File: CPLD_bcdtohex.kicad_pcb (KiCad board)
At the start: 2 copper layers, 27 x 90.1 mm, 5 parts, among them IC1 ATF750C-10PU, J1 Conn_01x08_Pin

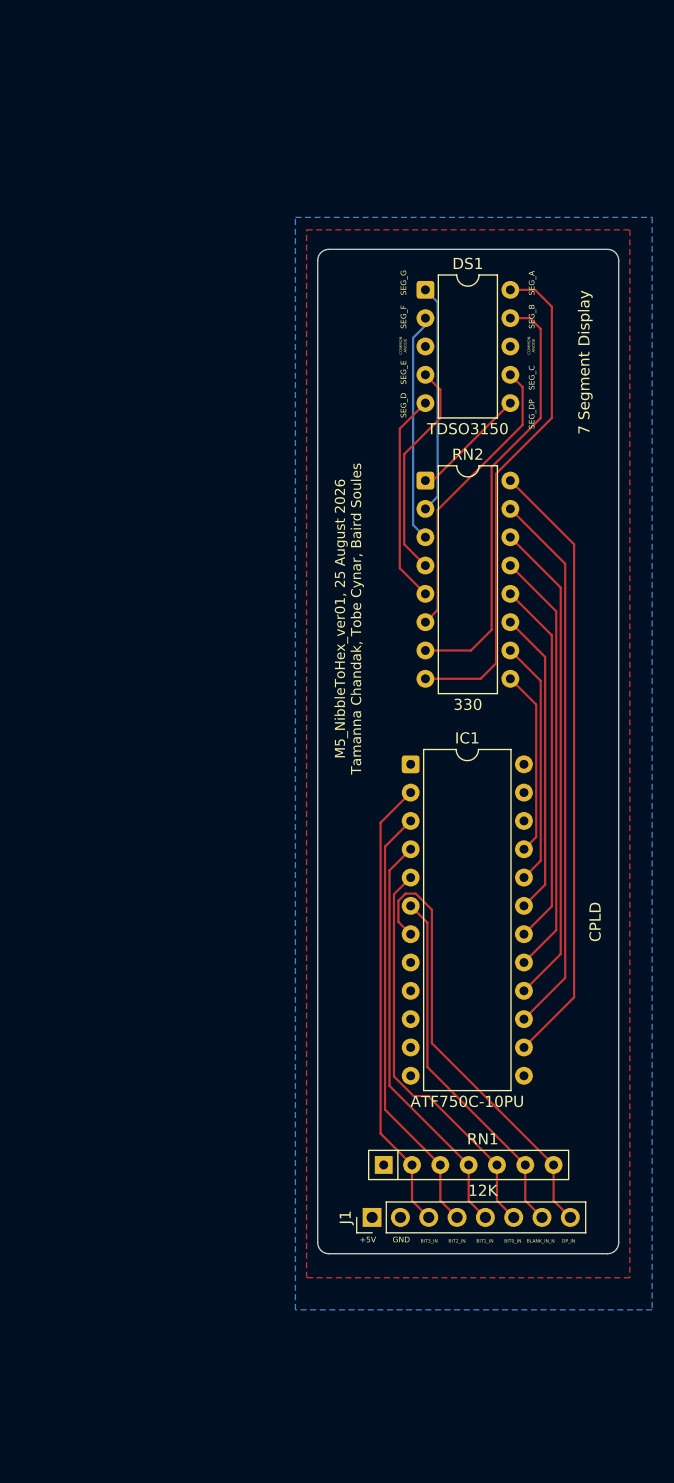
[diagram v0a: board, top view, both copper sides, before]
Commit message: PCB RevA
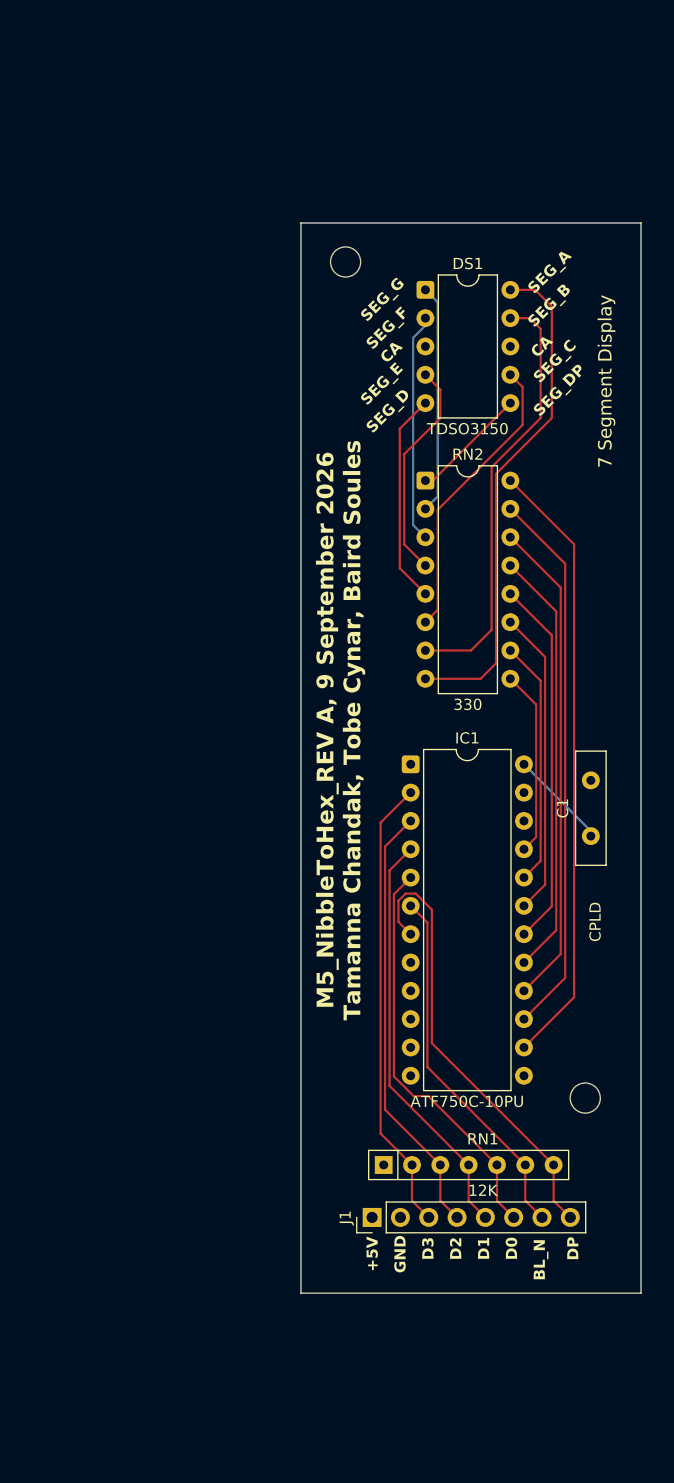
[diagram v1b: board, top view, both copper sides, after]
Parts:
- added C1: 0.1µF, Capacitor_THT:C_Disc_D10.0mm_W2.5mm_P5.00mm, F.Cu at (163.5, 114.5)
- added mh: MountingHole_2.7mm_M2.5, MountingHole:MountingHole_2.7mm_M2.5, F.Cu at (163.0, 138.0)
- added mh: MountingHole_2.7mm_M2.5, MountingHole:MountingHole_2.7mm_M2.5, F.Cu at (141.5, 63.0)
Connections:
- net /BIT1_IN renamed /D1
- net /BIT3_IN renamed /D3
- net /BLANK_IN_N renamed /BLANK
- net /DP_IN renamed /DP
- IC1 pad 24: +5V -> Net-(IC1-VCC)
- IC1 pad 3: /BIT2_IN -> /D2
- IC1 pad 5: /BIT2_IN -> /D0
- J1 pad 4: /BIT2_IN -> /D2
- J1 pad 6: /BIT2_IN -> /D0
- RN1 pad 3: /BIT2_IN -> /D2
- RN1 pad 5: /BIT2_IN -> /D0
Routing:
- net /BIT2_IN: track 75.6 -> 0.00 mm
- net /D2: track 0.00 -> 39.2 mm
- net /D0: track 0.00 -> 36.4 mm
- net Net-(IC1-VCC): track 0.00 -> 8.93 mm
- added copper zone on In1.Cu, net +5V
- added copper zone on In2.Cu, net GND
- removed copper zone on F.Cu, net +5V
- removed copper zone on B.Cu, net GND
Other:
- board size 27 x 90.1 mm -> 30.5 x 96 mm
- copper layers 2 -> 4
- board text added: "BL_N"
- board text added: "CA"
- board text added: "D0"
- board text added: "D1"
- board text added: "D2"
- board text added: "D3"
- board text added: "DP"
- board text added: "M5_NibbleToHex_REV A, 9 September 2026 Tamanna Chandak, Tobe Cynar, Baird Soules"
- board text added: "https://www.umassamherstm5.org/blog/m5hexdisplay"
- board text removed: "BIT0_IN"
- board text removed: "BIT1_IN"
- board text removed: "BIT2_IN"
- board text removed: "BIT3_IN"
- board text removed: "BLANK_IN_N"
- board text removed: "COMMON ANODE"
- board text removed: "DP_IN"
- board text removed: "M5_NibbleToHex_ver01, 25 August 2026 Tamanna Chandak, Tobe Cynar, Baird Soules"

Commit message: v0.5
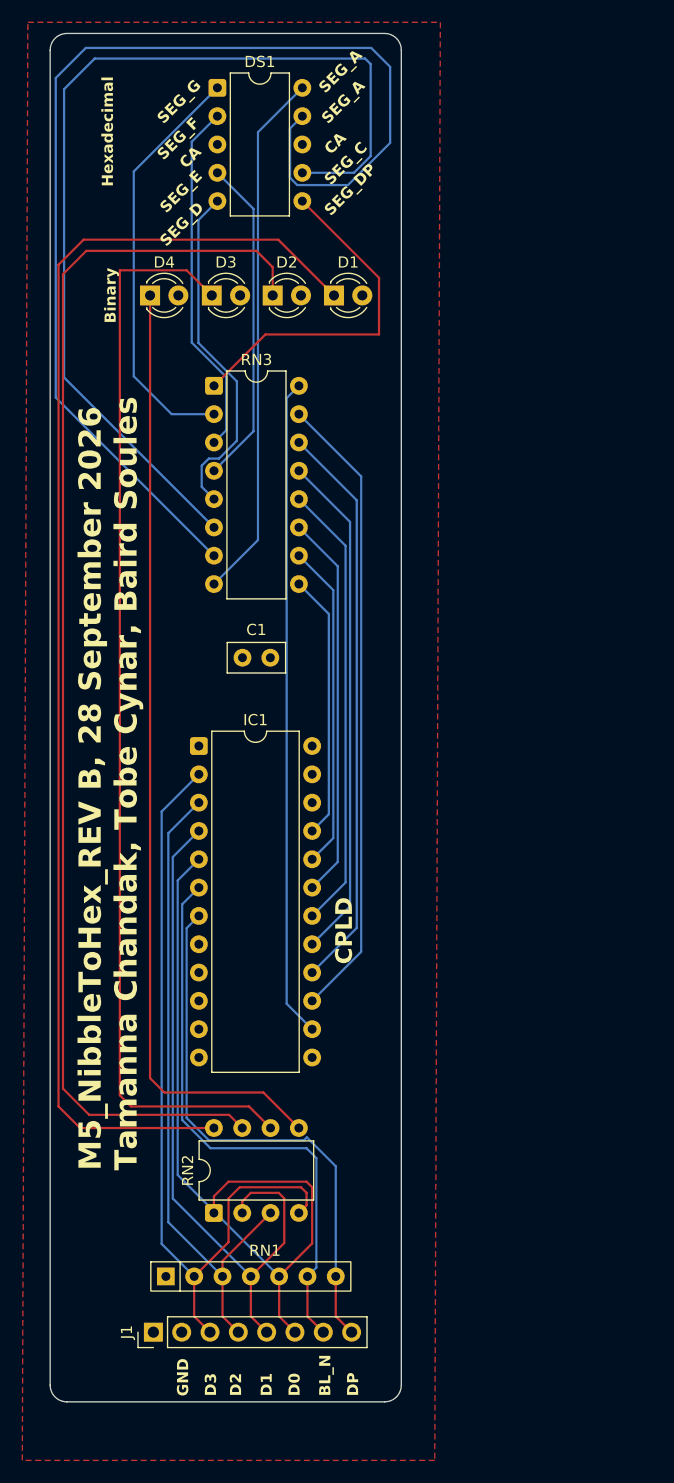
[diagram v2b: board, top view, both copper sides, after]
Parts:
- removed mh (x2): MountingHole_2.7mm_M2.5, MountingHole:MountingHole_2.7mm_M2.5
- added D1: LED, LED_THT:LED_D3.0mm, F.Cu at (140.5, 66.0)
- added D2: LED, LED_THT:LED_D3.0mm, F.Cu at (135.0, 66.0)
- added D3: LED, LED_THT:LED_D3.0mm, F.Cu at (129.5, 66.0)
- added D4: LED, LED_THT:LED_D3.0mm, F.Cu at (124.0, 66.0)
- added RN3: 330, Package_DIP:DIP-16_W7.62mm, F.Cu at (129.7, 74.1)
- C1: footprint Capacitor_THT:C_Disc_D10.0mm_W2.5mm_P5.00mm -> Capacitor_THT:C_Disc_D5.0mm_W2.5mm_P2.50mm
- RN1: value 12K -> 10K
- RN2: value 330 -> 220; footprint Package_DIP:DIP-16_W7.62mm -> Package_DIP:DIP-8_W7.62mm
- moved RN2 68.4 mm to (129.7, 148.3), turned to 90 degrees
- moved C1 35.1 mm to (132.2, 98.5), turned to 0 degrees
- moved DS1 26.0 mm to (130.0, 47.4)
- moved J1 22.2 mm to (124.3, 159.0)
- moved RN1 22.0 mm to (125.4, 154.0)
- moved IC1 19.1 mm to (128.3, 106.4)
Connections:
- net /BLANK renamed /BLANK_N
- C1 pad 1: Net-(IC1-VCC) -> +5V
- IC1 pad 24: Net-(IC1-VCC) -> +5V
- RN2 pad 1: Net-(DS1-DP) -> /D0
- RN2 pad 2: Net-(DS1-g) -> /D1
- RN2 pad 3: Net-(DS1-f) -> /D2
- RN2 pad 4: Net-(DS1-e) -> /D3
- RN2 pad 5: Net-(DS1-d) -> Net-(D4-K)
- RN2 pad 6: Net-(DS1-c) -> Net-(D3-K)
- RN2 pad 7: Net-(DS1-b) -> Net-(D2-K)
- RN2 pad 8: Net-(DS1-a) -> Net-(D1-K)
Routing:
- net Net-(D1-K): track 0.00 -> 118.0 mm
- net Net-(D2-K): track 0.00 -> 113.4 mm
- net Net-(D3-K): track 0.00 -> 97.9 mm
- net Net-(D4-K): track 0.00 -> 85.4 mm
- net Net-(DS1-b): track 38.6 -> 104.2 mm
- net Net-(DS1-c): track 26.3 -> 88.7 mm
- net /D0: track 36.4 -> 67.8 mm
- net /D3: track 41.0 -> 71.2 mm
- net /D1: track 37.4 -> 63.0 mm
- net Net-(DS1-DP): track 10.5 -> 31.5 mm
- net /D2: track 39.2 -> 58.7 mm
- net /BLANK_N: track 32.8 -> 51.5 mm
- net Net-(DS1-g): track 20.6 -> 37.6 mm
- net Net-(DS1-d): track 19.0 -> 31.2 mm
- net Net-(DS1-f): track 21.6 -> 32.0 mm
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- added copper zone on F.Cu, net +5V
- removed copper zone on In1.Cu, net +5V
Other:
- board size 30.5 x 96 mm -> 31.5 x 122.8 mm
- board text added: "Binary"
- board text added: "Hexadecimal"
- board text added: "M5_NibbleToHex_REV B, 28 September 2026 Tamanna Chandak, Tobe Cynar, Baird Soules"
- board text removed: "+5V"
- board text removed: "7 Segment Display"
- board text removed: "M5_NibbleToHex_REV A, 9 September 2026 Tamanna Chandak, Tobe Cynar, Baird Soules"
- board text removed: "SEG_B"
